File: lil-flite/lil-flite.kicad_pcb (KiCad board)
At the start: 2 copper layers, 25 x 50 mm, 25 parts, among them J201 USB4105-GF-A, J202 Conn_01x02, J203 Conn_01x02, J204 Conn_02x06_Odd_Even, T201 AO3401A, U301 BMP280, U302 MC6470, U501 STM32F103C8T6

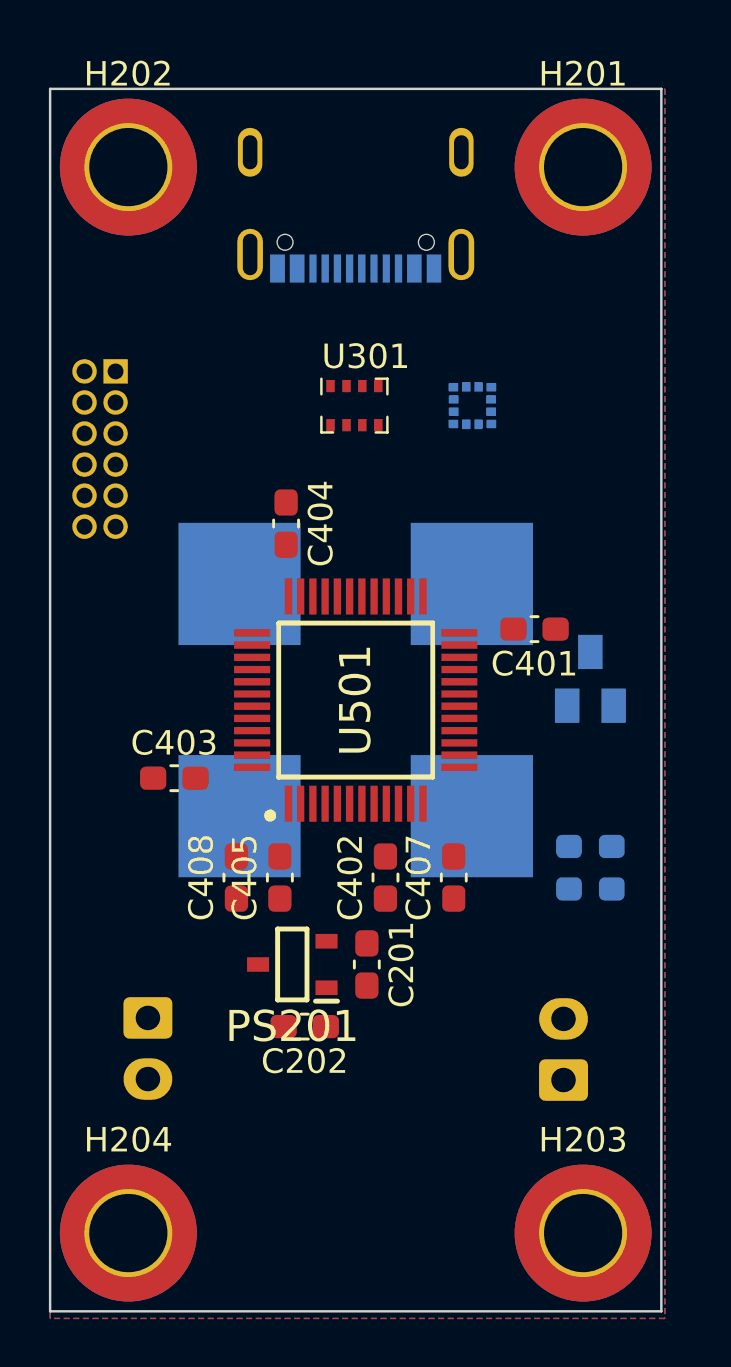
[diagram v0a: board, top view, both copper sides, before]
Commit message: aaa
adding buttons
changin layout
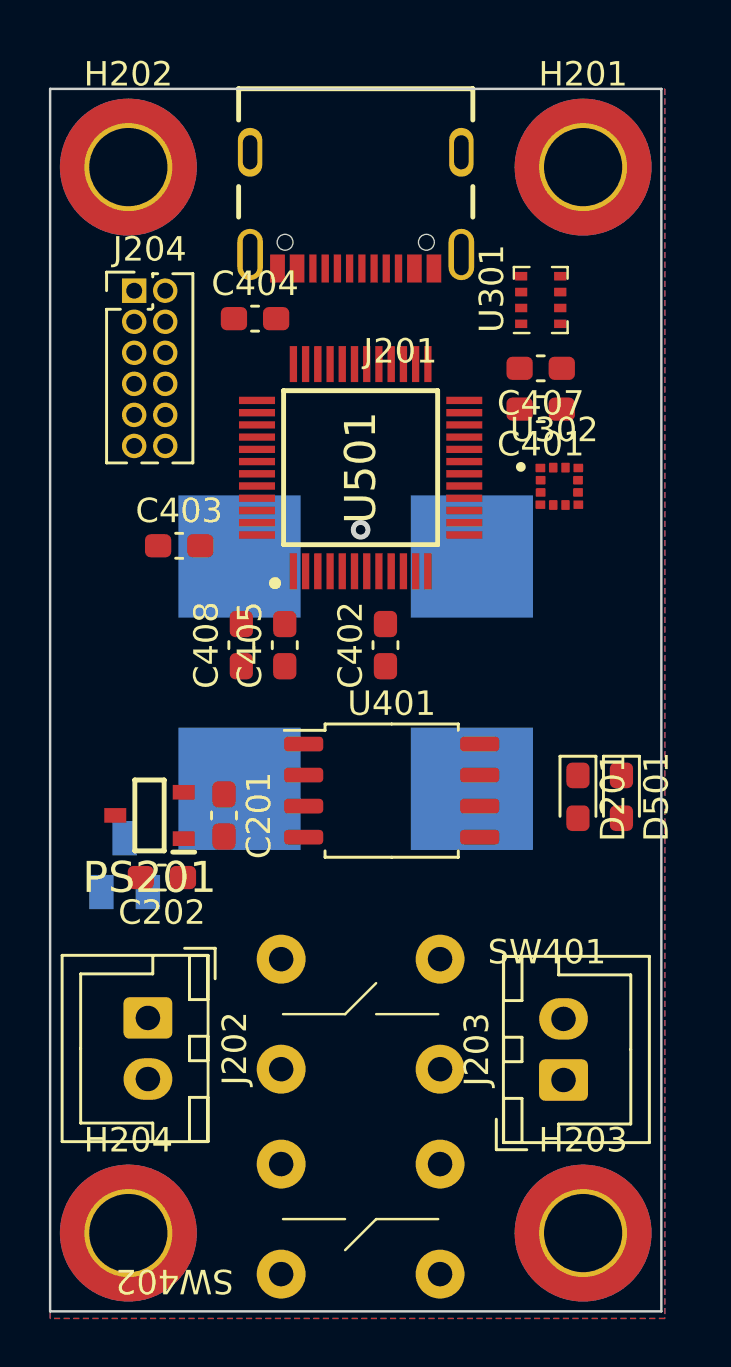
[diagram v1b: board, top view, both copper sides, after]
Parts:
- added SW401: PTS645SM70-2 LFS, lil-flite:PTS645SM70-2 LFS, F.Cu at (112.7, 87.8)
- added SW402: PTS645SM70-2 LFS, lil-flite:PTS645SM70-2 LFS, F.Cu at (112.7, 96.2)
- added U401: W25Q128JVSIQ, Package_SO:SOIC-8_5.23x5.23mm_P1.27mm, F.Cu at (114.0, 78.7)
- D201, D501, J201, J202, J203, J204, U302: moved to F.Cu
- moved C407 21.1 mm to (120.1, 61.4), turned to 180 degrees
- moved T201 20.5 mm to (103.0, 81.8)
- moved C403 9.51 mm to (105.3, 68.7)
- moved C405 9.51 mm to (109.6, 72.8)
- moved C408 9.51 mm to (107.8, 72.8)
- moved U501 9.51 mm to (112.7, 65.5)
- moved C402 9.51 mm to (113.7, 72.8)
- moved C401 9.00 mm to (120.1, 63.1)
- moved U301 8.76 mm to (120.1, 58.6), turned to 90 degrees
- moved C404 8.48 mm to (108.4, 59.4), turned to 0 degrees
- moved PS201 8.44 mm to (104.1, 79.7)
- moved C202 8.44 mm to (104.6, 82.3)
- moved C201 8.44 mm to (107.1, 79.7)
- moved U302 4.85 mm to (120.8, 66.3), turned to 0 degrees
- moved D501 3.98 mm to (123.4, 79.0), turned to -90 degrees
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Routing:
- net GND: vias 0 -> 1
- added copper zone on In1.Cu, net GND
- added copper zone on In2.Cu, net GND
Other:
- copper layers 2 -> 4

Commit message: Almost finished
Need to double check everything
routing done
more vias maybe
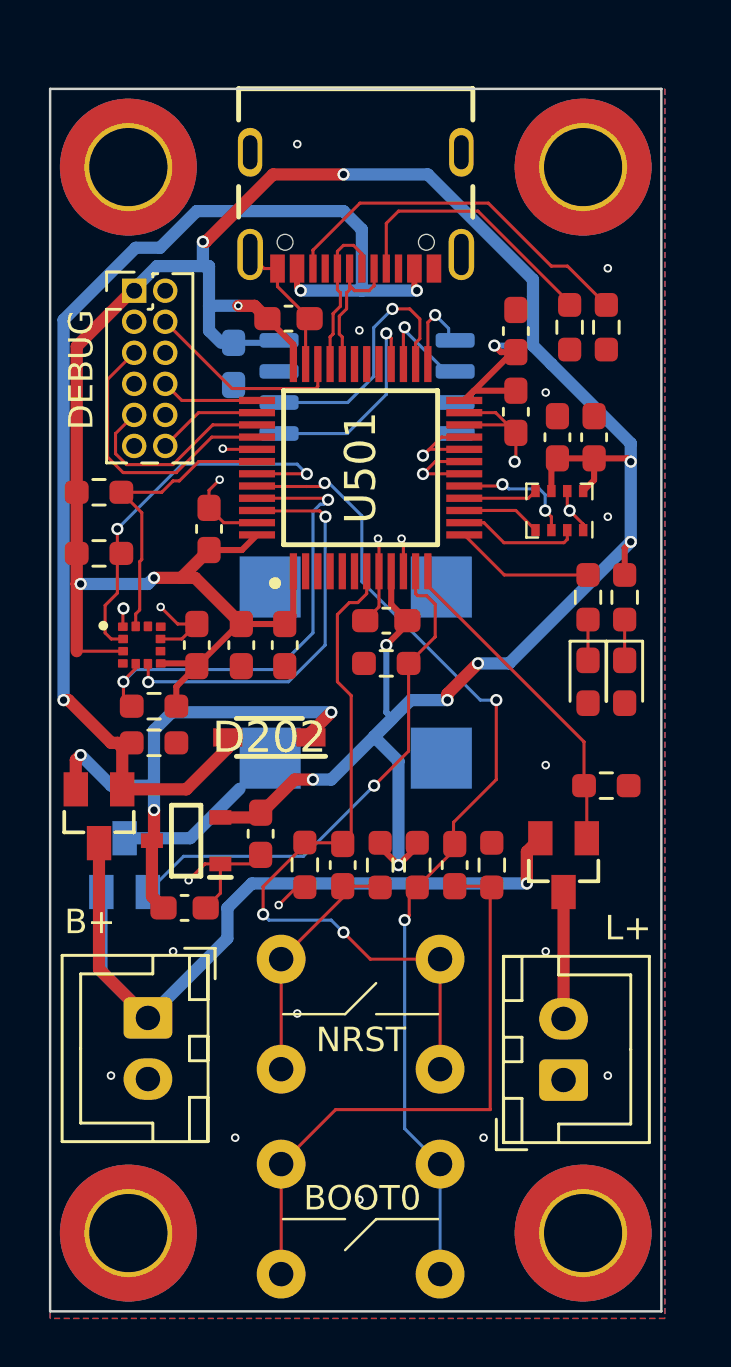
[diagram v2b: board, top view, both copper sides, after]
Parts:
- added C301: 100nF, Capacitor_SMD:C_0603_1608Metric_Pad1.08x0.95mm_HandSolder, F.Cu at (106.0, 72.8)
- added C302: 100nF, Capacitor_SMD:C_0603_1608Metric_Pad1.08x0.95mm_HandSolder, F.Cu at (120.8, 64.2)
- added C303: 100nF, Capacitor_SMD:C_0603_1608Metric_Pad1.08x0.95mm_HandSolder, F.Cu at (122.2, 64.2)
- added C406: 100nF, Capacitor_SMD:C_0603_1608Metric_Pad1.08x0.95mm_HandSolder, F.Cu at (112.0, 81.7)
- added C409: 100nF, Capacitor_SMD:C_0603_1608Metric_Pad1.08x0.95mm_HandSolder, F.Cu at (116.5, 81.7)
- added C410: 100nF, Capacitor_SMD:C_0603_1608Metric_Pad1.08x0.95mm_HandSolder, B.Cu at (107.5, 61.2)
- added D202: 1N4148W-7-F, SamacSys_Parts:SOD3716X145N, F.Cu at (109.0, 76.5)
- added R201: 330R, Resistor_SMD:R_0603_1608Metric_Pad0.98x0.95mm_HandSolder, F.Cu at (123.5, 70.8)
- added R202: 10k, Resistor_SMD:R_0603_1608Metric_Pad0.98x0.95mm_HandSolder, F.Cu at (113.8, 73.5)
- added R203: 10k, Resistor_SMD:R_0603_1608Metric_Pad0.98x0.95mm_HandSolder, F.Cu at (122.8, 78.5)
- added R204: 1k, Resistor_SMD:R_0603_1608Metric_Pad0.98x0.95mm_HandSolder, F.Cu at (104.2, 76.8)
- added R205: 5k1, Resistor_SMD:R_0603_1608Metric_Pad0.98x0.95mm_HandSolder, F.Cu at (121.2, 59.8)
- added R206: 5k1, Resistor_SMD:R_0603_1608Metric_Pad0.98x0.95mm_HandSolder, F.Cu at (122.8, 59.8)
- added R301: 4k7, Resistor_SMD:R_0603_1608Metric_Pad0.98x0.95mm_HandSolder, F.Cu at (102.0, 69.0)
- added R302: 4k7, Resistor_SMD:R_0603_1608Metric_Pad0.98x0.95mm_HandSolder, F.Cu at (102.0, 66.5)
- added R303: 4k7, Resistor_SMD:R_0603_1608Metric_Pad0.98x0.95mm_HandSolder, F.Cu at (104.2, 75.2)
- added R401: 1k, Resistor_SMD:R_0603_1608Metric_Pad0.98x0.95mm_HandSolder, F.Cu at (113.5, 81.8)
- added R402: 1k, Resistor_SMD:R_0603_1608Metric_Pad0.98x0.95mm_HandSolder, F.Cu at (118.1, 81.7)
- added R405: 10k, Resistor_SMD:R_0603_1608Metric_Pad0.98x0.95mm_HandSolder, F.Cu at (115.0, 81.7)
- added R406: 10k, Resistor_SMD:R_0603_1608Metric_Pad0.98x0.95mm_HandSolder, F.Cu at (110.4, 81.7)
- added R407: 330R, Resistor_SMD:R_0603_1608Metric_Pad0.98x0.95mm_HandSolder, F.Cu at (122.0, 70.8)
- added T202: AO3401A, JLC-Transistors:SOT23-3L, F.Cu at (102.0, 79.8)
- added T203: AO3401A, JLC-Transistors:SOT23-3L, F.Cu at (121.0, 81.8)
- BZ201: value Buzzer -> CMT-8504-100-SMT-TR; footprint lil-flite:CMT-8504-100-SMT-TR -> lil-flite:XDCR_CMT-8504-100-SMT-TR
- U401: moved to B.Cu
- moved U302 18.3 mm to (103.8, 72.8)
- moved U401 16.5 mm to (113.0, 62.2), turned to 180 degrees
- moved U301 8.65 mm to (120.8, 67.2), turned to 180 degrees
- moved D201 5.08 mm to (123.5, 74.2)
- moved D501 4.90 mm to (122.0, 74.2)
- moved C407 1.83 mm to (119.0, 59.9), turned to -90 degrees
- moved PS201 1.82 mm to (105.6, 80.8)
- moved C201 1.68 mm to (108.6, 80.5), turned to 90 degrees
- moved C202 1.55 mm to (105.5, 83.5)
- moved C403 1.40 mm to (106.5, 68.0), turned to -90 degrees
- moved C404 1.37 mm to (109.8, 59.4), turned to 180 degrees
- moved C401 1.02 mm to (119.0, 63.2), turned to 90 degrees
- moved C402 1.00 mm to (113.8, 71.8), turned to 0 degrees
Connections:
- BZ201 pad 1: Net-(BZ201--) -> (no net)
- BZ201 pad 2: GND -> (no net)
- C202 pad 2: +BATT -> Net-(C202--)
- D201 pad 1: unconnected-(D201-K-Pad1) -> Net-(D201-K)
- D201 pad 2: unconnected-(D201-A-Pad2) -> GND
- D501 pad 1: unconnected-(D501-K-Pad1) -> Net-(D501-K)
- D501 pad 2: unconnected-(D501-A-Pad2) -> GND
- PS201 pad 3: +BATT -> Net-(C202--)
- SW401 pad 2: Net-(SW401-Pad2) -> /MCU/MCU_NRST
- SW401 pad 4: Net-(SW401-Pad2) -> /MCU/MCU_NRST
- SW402 pad 1: Net-(SW402-Pad1) -> /MCU/MCU_BOOT0
- SW402 pad 3: Net-(SW402-Pad1) -> /MCU/MCU_BOOT0
- T201 pad 1: unconnected-(T201-Pad1) -> /Connectors + Power/MISC.Buzzer_PWM
- U301 pad 1: unconnected-(U301-GND-Pad1) -> GND
- U301 pad 2: unconnected-(U301-CSB-Pad2) -> /MCU/BMP.NSS
- U301 pad 3: unconnected-(U301-SDI-Pad3) -> /MCU/BMP.MOSI
- U301 pad 4: unconnected-(U301-SCK-Pad4) -> /MCU/BMP.SCK
- U301 pad 5: unconnected-(U301-SDO-Pad5) -> /MCU/BMP.MISO
- U301 pad 6: unconnected-(U301-VDDIO-Pad6) -> VCC
- U301 pad 7: unconnected-(U301-GND-Pad7) -> GND
- U301 pad 8: unconnected-(U301-VDD-Pad8) -> VCC
- U302 pad 1: unconnected-(U302-A5-Pad1) -> GND
- U302 pad 12: unconnected-(U302-SCL-Pad12) -> /MCU/IMU.SCL
- U302 pad 2: unconnected-(U302-SDA-Pad2) -> /MCU/IMU.SDA
- U302 pad 3: unconnected-(U302-VDDIO-Pad3) -> VCC
- U302 pad 5: unconnected-(U302-INTA-Pad5) -> /MCU/IMU.INTA
- U302 pad 6: unconnected-(U302-INTM-Pad6) -> /MCU/IMU.INTM
- U302 pad 7: unconnected-(U302-VDDM-Pad7) -> VCC
- U302 pad 9: unconnected-(U302-GND-Pad9) -> GND
- U401 pad 1: unconnected-(U401-~{CS}-Pad1) -> /MCU/FLASH.NSS
- U401 pad 2: unconnected-(U401-DO(IO1)-Pad2) -> /MCU/FLASH.MISO
- U401 pad 4: unconnected-(U401-GND-Pad4) -> GND
- U401 pad 5: unconnected-(U401-DI(IO0)-Pad5) -> /MCU/FLASH.MOSI
- U401 pad 6: unconnected-(U401-CLK-Pad6) -> /MCU/FLASH.SCK
- U401 pad 8: unconnected-(U401-VCC-Pad8) -> VCC
- U501 pad 10: unconnected-(U501-PA0_WKUP-Pad10) -> GND
- U501 pad 11: unconnected-(U501-PA1-Pad11) -> /Connectors + Power/MISC.Buzzer_PWM
- U501 pad 12: unconnected-(U501-PA2-Pad12) -> /Connectors + Power/MISC.RECOVERY_LED_PWM
- U501 pad 13: unconnected-(U501-PA3-Pad13) -> /MCU/MCU_GPLED
- U501 pad 14: unconnected-(U501-PA4-Pad14) -> /MCU/BMP.NSS
- U501 pad 15: unconnected-(U501-PA5-Pad15) -> /MCU/BMP.SCK
- U501 pad 16: unconnected-(U501-PA6-Pad16) -> /MCU/BMP.MISO
- U501 pad 17: unconnected-(U501-PA7-Pad17) -> /MCU/BMP.MOSI
- U501 pad 18: unconnected-(U501-PB0-Pad18) -> GND
- U501 pad 19: unconnected-(U501-PB1-Pad19) -> GND
- U501 pad 2: unconnected-(U501-PC13-TAMPER-RTC-Pad2) -> GND
- U501 pad 20: unconnected-(U501-PB2-Pad20) -> GND
- U501 pad 21: unconnected-(U501-PB10-Pad21) -> GND
- U501 pad 22: unconnected-(U501-PB11-Pad22) -> GND
- U501 pad 25: unconnected-(U501-PB12-Pad25) -> /MCU/FLASH.NSS
- U501 pad 26: unconnected-(U501-PB13-Pad26) -> /MCU/FLASH.SCK
- U501 pad 27: unconnected-(U501-PB14-Pad27) -> /MCU/FLASH.MISO
- U501 pad 28: unconnected-(U501-PB15-Pad28) -> /MCU/FLASH.MOSI
- U501 pad 29: unconnected-(U501-PA8-Pad29) -> GND
- U501 pad 3: unconnected-(U501-PC14-OSC32_IN-Pad3) -> GND
- U501 pad 30: unconnected-(U501-PA9-Pad30) -> GND
- U501 pad 31: unconnected-(U501-PA10-Pad31) -> GND
- U501 pad 32: /MCU/USB.Data_- -> /Connectors + Power/USB.Data_-
- U501 pad 33: /MCU/USB.Data_+ -> /Connectors + Power/USB.Data_+
- U501 pad 34: /MCU/JTAG.MSSWDIO -> /Connectors + Power/JTAG.MSSWDIO
- U501 pad 39: /MCU/JTAG.DOSWO -> /Connectors + Power/JTAG.DOSWO
- U501 pad 4: unconnected-(U501-PC15-OSC32_OUT-Pad4) -> GND
- U501 pad 41: unconnected-(U501-PB5-Pad41) -> GND
- U501 pad 42: unconnected-(U501-PB6-Pad42) -> /MCU/IMU.SCL
- U501 pad 43: unconnected-(U501-PB7-Pad43) -> /MCU/IMU.SDA
- U501 pad 44: unconnected-(U501-BOOT0-Pad44) -> /MCU/MCU_BOOT0
- U501 pad 45: unconnected-(U501-PB8-Pad45) -> /MCU/IMU.INTA
- U501 pad 46: unconnected-(U501-PB9-Pad46) -> /MCU/IMU.INTM
- U501 pad 5: unconnected-(U501-PD0_OSC_IN-Pad5) -> GND
- U501 pad 6: unconnected-(U501-PD1_OSC_OUT-Pad6) -> GND
- U501 pad 7: unconnected-(U501-NRST-Pad7) -> /MCU/MCU_NRST
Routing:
- net VCC: track 0.00 -> 135.7 mm, vias 0 -> 13
- net +5V: track 0.00 -> 51.2 mm, vias 0 -> 3
- net GND: track 0.00 -> 42.0 mm, vias 1 -> 26
- net /MCU/MCU_BOOT0: track 0.00 -> 40.7 mm, vias 0 -> 3
- net +BATT: track 0.00 -> 34.5 mm, vias 0 -> 1
- net /MCU/MCU_NRST: track 0.00 -> 29.9 mm, vias 0 -> 2
- net Net-(C409-+): track 0.00 -> 24.6 mm
- net Net-(C202--): track 0.00 -> 21.4 mm, vias 0 -> 3
- net /Connectors + Power/MISC.Buzzer_PWM: track 0.00 -> 21.4 mm, vias 0 -> 1
- net /MCU/IMU.INTA: track 0.00 -> 19.6 mm, vias 0 -> 2
- net /MCU/IMU.INTM: track 0.00 -> 16.8 mm, vias 0 -> 2
- net /MCU/IMU.SDA: track 0.00 -> 16.3 mm, vias 0 -> 2
- net /Connectors + Power/USB.CC2: track 0.00 -> 15.3 mm
- net /Connectors + Power/MISC.RECOVERY_LED_PWM: track 0.00 -> 13.6 mm
- net /MCU/IMU.SCL: track 0.00 -> 12.0 mm
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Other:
- board text added: "B+"
- board text added: "BOOT0"
- board text added: "CL"
- board text added: "DEBUG"
- board text added: "DI"
- board text added: "L+"
- board text added: "NRST"
- board text added: "RST"
- board text added: "SW"
- board text added: "SWO"
- board text added: "VCC"
